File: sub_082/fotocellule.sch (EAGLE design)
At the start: 39 parts, among them IC1 TL082P, IC3 NE555N, IC5 7805TV, IC6 NE555N, Q1 2N3904, T1 BD647

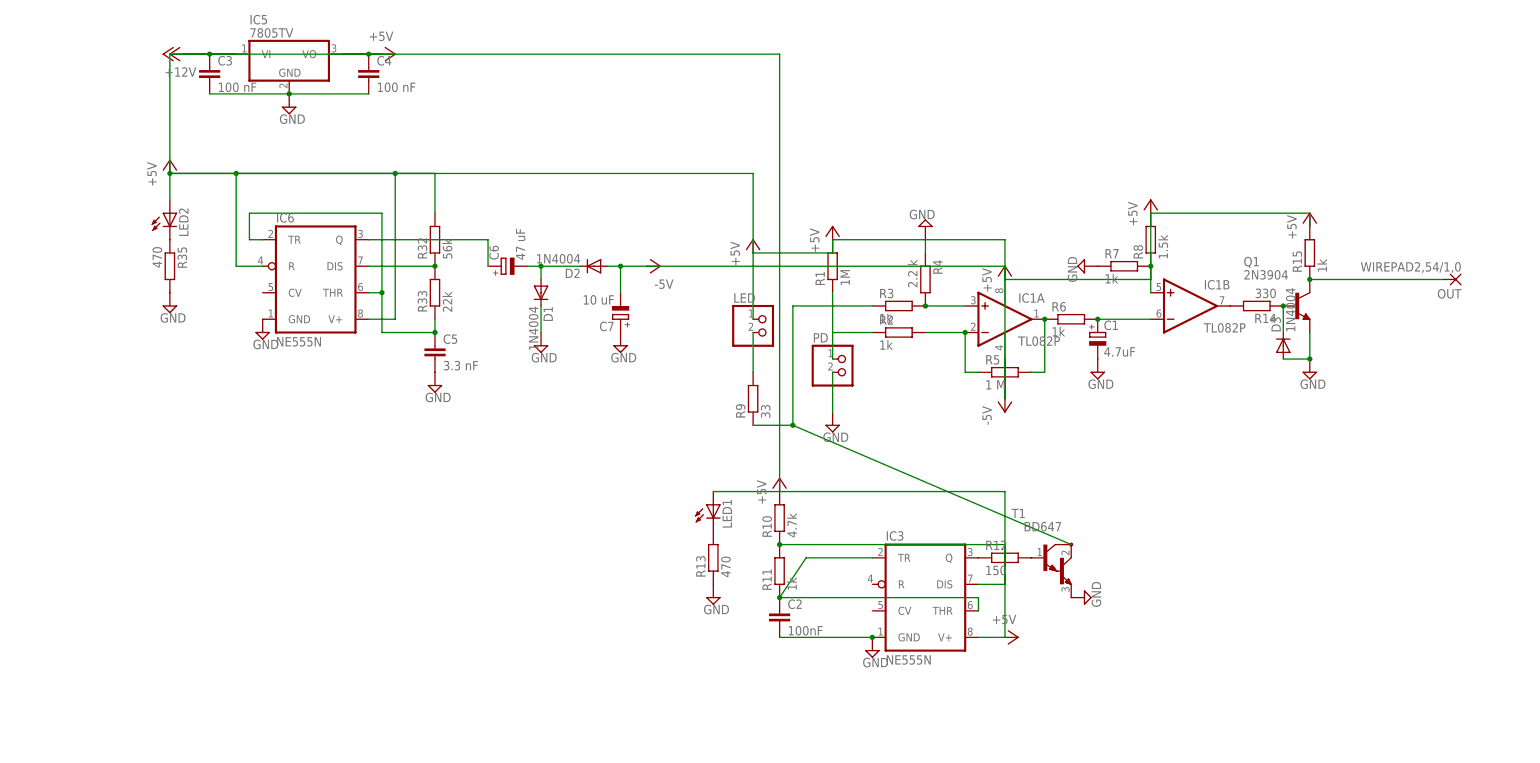
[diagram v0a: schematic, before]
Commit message: Rewired correctly sub082
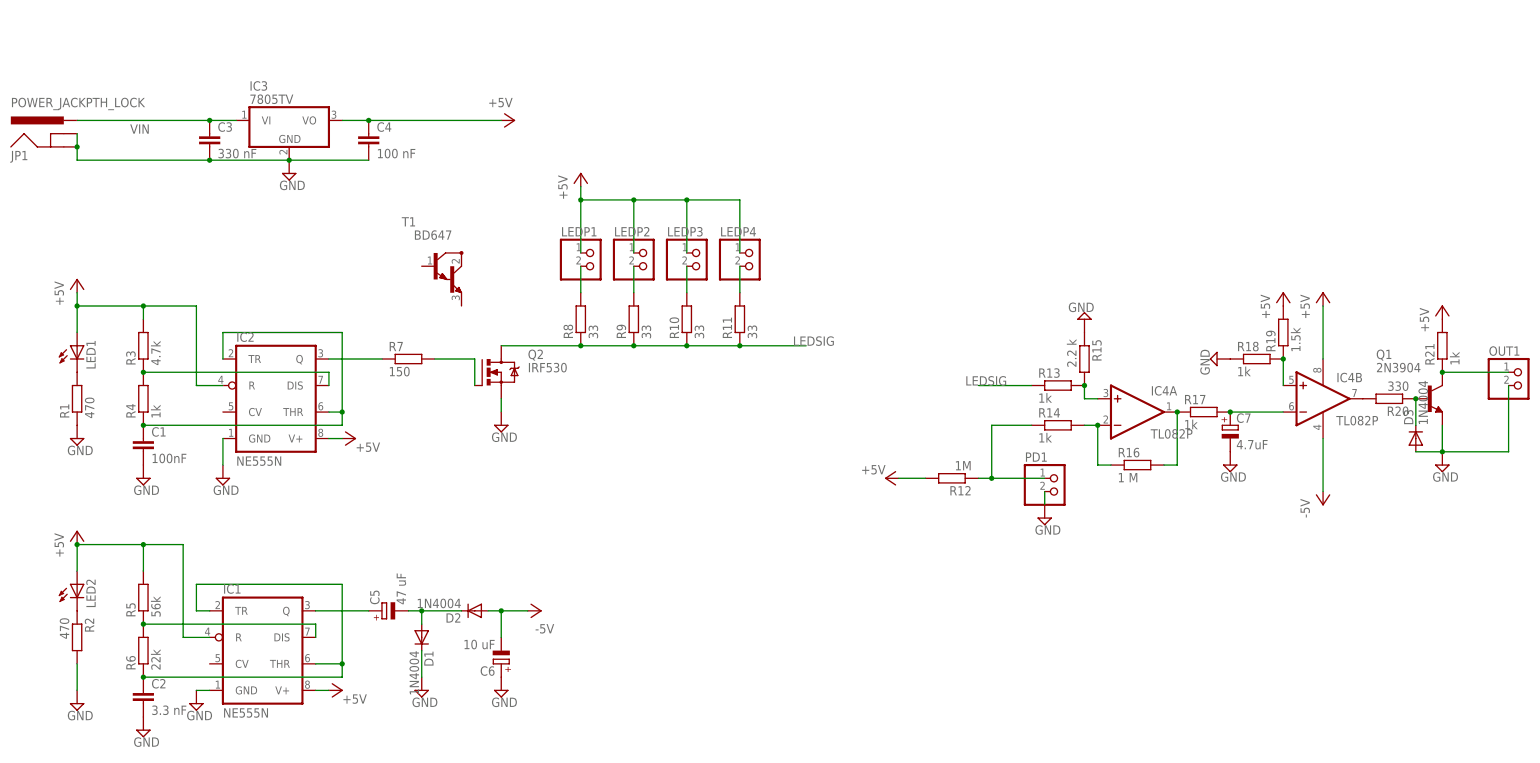
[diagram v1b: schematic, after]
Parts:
- removed IC5: 7805TV, linear:7805TV
- removed IC6: NE555N, linear:NE555N
- removed LED, PD: (no value), pinhead:PINHD-1X2
- removed OUT: WIREPAD2,54/1,0, wirepad:WIREPAD2,54/1,0
- removed R32: 56k, resistor:R-EU_0207/10
- removed R33: 22k, resistor:R-EU_0207/10
- removed R35: 470, resistor:R-EU_0207/10
- added IC2: NE555N, linear:NE555N
- added IC4: TL082P, linear:TL082P
- added JP1: POWER_JACKPTH_LOCK, SparkFun-Connectors:POWER_JACKPTH_LOCK
- added LEDP1, LEDP2, LEDP3, LEDP4, OUT1, PD1: (no value), pinhead:PINHD-1X2
- added Q2: IRF530, transistor-power:IRF530
- added R16: 1 M, resistor:R-EU_0207/10
- added R17, R18, R21: 1k, resistor:R-EU_0207/10
- added R19: 1.5k, resistor:R-EU_0207/10
- added R20: 330, resistor:R-EU_0207/10
- C1: value 4.7uF -> 100nF; device resistor:CPOL-EUE2.5-6 -> resistor:C-EU025-024X044
- C2: value 100nF -> 3.3 nF
- C3: value 100 nF -> 330 nF
- C5: value 3.3 nF -> 47 uF; device resistor:C-EU025-024X044 -> rcl:CPOL-EUE2.5-5
- C6: value 47 uF -> 10 uF
- C7: value 10 uF -> 4.7uF; device rcl:CPOL-EUE2.5-5 -> resistor:CPOL-EUE2.5-6
- IC1: value TL082P -> NE555N; device linear:TL082P -> linear:NE555N
- IC3: value NE555N -> 7805TV; device linear:NE555N -> linear:7805TV
- R1: value 1M -> 470
- R10: value 4.7k -> 33
- R11: value 1k -> 33
- R12: value 150 -> 1M
- R13: value 470 -> 1k
- R14: value 330 -> 1k
- R15: value 1k -> 2.2 k
- R2: value 1k -> 470
- R3: value 1k -> 4.7k
- R4: value 2.2 k -> 1k
- R5: value 1 M -> 56k
- R6: value 1k -> 22k
- R7: value 1k -> 150
- R8: value 1.5k -> 33
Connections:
- removed net N$33: C6.+, IC6.Q
- removed net N$34: C5.1, IC6.THR, IC6.TR, R33.1
- removed net N$35: C6.-, D1.A, D2.C
- removed net VCC: C3.1, IC5.VI
- new net LEDSIG: Q2.D, R10.1, R11.1, R13.1, R8.1, R9.1
- new net N$11: C5.-, D1.A, D2.C
- new net N$17: LEDP2.2, R9.2
- new net N$19: LEDP3.2, R10.2
- new net N$20: LEDP4.2, R11.2
- new net N$21: IC4A.-IN, R14.2, R16.1
- new net VIN: C3.1, IC3.VI, JP1.PWR
- net +5V: now also IC1.R, IC1.V+, IC2.R, IC2.V+, IC3.VO, IC4P.V+, LEDP1.1, LEDP2.1, LEDP3.1, LEDP4.1, R12.2, R19.2, R21.2, R3.2, R5.2; no longer IC1P.V+, IC3.V+, IC5.VO, IC6.R, IC6.V+, LED.1, R1.2, R10.2, R15.2, R32.2, R8.2
- net -5V: now also C6.-, IC4P.V-; no longer C7.-, IC1P.V-
- net GND: now also C1.2, C6.+, C7.-, IC1.GND, IC2.GND, JP1.GND, JP1.GNDBREAK, OUT1.2, PD1.2, Q2.S, R1.1, R15.1, R18.1, R2.2; no longer C1.-, C5.2, C7.+, IC5.GND, IC6.GND, PD.2, R13.1, R35.2, R4.1, R7.1, T1.E
- net N$1: now also C1.1, IC2.THR, IC2.TR, R4.1; no longer PD.1, R1.1, R2.1
- net N$10: now also C5.+, IC1.Q; no longer C2.1, IC3.THR, IC3.TR, R11.1
- net N$12: now also Q2.G, R7.2; no longer R12.2, T1.B
- net N$13: now also IC4B.OUT, R20.2; no longer IC1B.OUT, R14.2
- net N$14: now also R1.2; no longer R13.2
- net N$15: now also LEDP1.2, R8.2; no longer IC3.DIS, R10.1, R11.2
- net N$16: now also OUT1.1, R21.1; no longer OUT.P, R15.1
- net N$18: now also R20.1; no longer R14.1
- net N$2: now also IC2.DIS, R3.1, R4.2; no longer IC1A.-IN, R2.2, R5.1
- net N$22: now also PD1.1, R12.1, R14.1; no longer R3.1, R9.1, T1.C
- net N$3: now also IC4A.+IN, R13.2, R15.2; no longer IC1A.+IN, R3.2, R4.2
- net N$32: now also R2.1; no longer R35.1
- net N$4: now also IC4A.OUT, R16.2, R17.1; no longer IC1A.OUT, R5.2, R6.1
- net N$5: now also C7.+, IC4B.-IN, R17.2; no longer C1.+, IC1B.-IN, R6.2
- net N$6: now also IC4B.+IN, R18.2, R19.1; no longer IC1B.+IN, R7.2, R8.1
- net N$7: now also C2.1, IC1.THR, IC1.TR, R6.1; no longer LED.2, R9.2
- net N$8: now also IC1.DIS, R5.1, R6.2; no longer IC6.DIS, R32.1, R33.2
- net N$9: now also IC2.Q, R7.1; no longer IC3.Q, R12.1
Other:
- moved on the sheet: C2, C3, C4, C6, C7, D1, D2, D3, LED1, LED2, Q1, R1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
